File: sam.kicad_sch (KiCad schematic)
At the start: 23 parts, among them IC4 74ACT02, IC5 74ACT138, IC6 74ACT138N, J1 JTAG, J3 Conn_01x24, J4 Conn_01x24, U3 XC95144XL-TQ100, X1 14.31818MHz

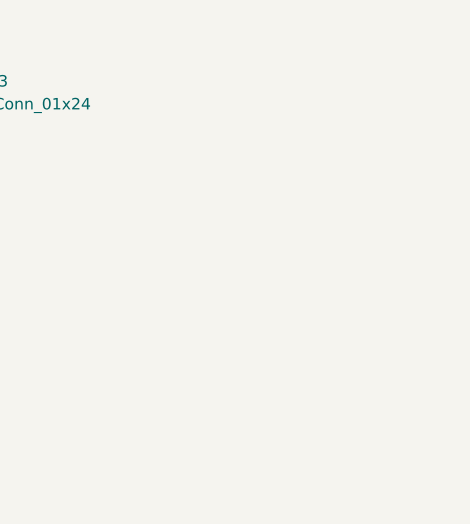
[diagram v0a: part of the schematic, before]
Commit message: progress routing
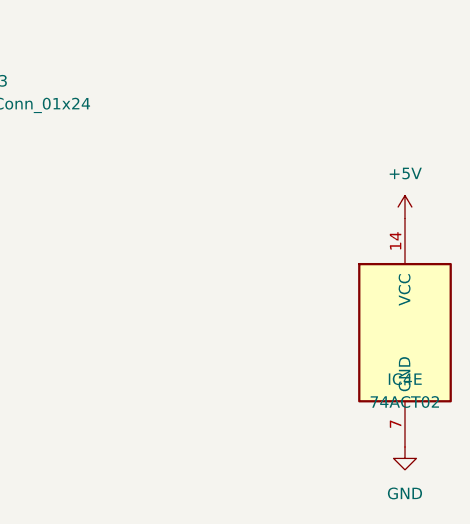
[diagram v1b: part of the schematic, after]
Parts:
- added unit 5 of IC4
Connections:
- net +5V: now also IC4.14 (VCC)
- net GND: now also IC4.7 (GND)
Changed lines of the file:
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@@
+	)
+	(symbol
+		(lib_id "74xx:74LS02")
+		(at 377.19 214.63 0)
+		(unit 5)
+		(exclude_from_sim no)
+		(in_bom yes)
+		(on_board yes)
+		(dnp no)
+		(property "Reference" "IC4"
+			(at 377.19 219.837 0)
+			(effects
+				(font
+					(size 1.27 1.27)
+				)
+			)
+		)
+		(property "Value" "74ACT02"
+			(at 377.19 222.377 0)
+			(effects
+				(font
+					(size 1.27 1.27)
+				)
+			)
+		)
+		(property "Footprint" "Package_SO:SOIC-14_3.9x8.7mm_P1.27mm"
+			(at 377.19 214.63 0)
+			(effects
+				(font
+					(size 1.27 1.27)
+				)
+				(hide yes)
+			)
+		)
+		(property "Datasheet" "http://www.ti.com/lit/gpn/sn74ls02"
+			(at 377.19 214.63 0)
+			(effects
+				(font
+					(size 1.27 1.27)
+				)
+				(hide yes)
+			)
+		)
+		(property "Description" ""
+			(at 377.19 214.63 0)
+			(effects
+				(font
+					(size 1.27 1.27)
+				)
+				(hide yes)
+			)
+		)
+		(property "DigiKey" "MC74ACT02DR2GOSCT-ND"
+			(at 377.19 214.63 0)
+			(effects
+				(font
+					(size 1.27 1.27)
+				)
+				(hide yes)
+			)
+		)
+		(property "SA2120" "Sheet 1 (spare)"
+			(at 377.19 214.63 0)
+			(effects
+				(font
+					(size 1.27 1.27)
+				)
+				(hide yes)
+			)
+		)
+		(pin "1"
+		)
+		(pin "2"
+		)
+		(pin "3"
+		)
+		(pin "4"
+		)
+		(pin "5"
+		)
+		(pin "6"
+		)
+		(pin "10"
+		)
+		(pin "8"
+		)
+		(pin "9"
+		)
+		(pin "11"
+		)
+		(pin "12"
+		)
+		(pin "13"
+		)
+		(pin "14"
+		)
+		(pin "7"
+		)
+		(instances
+			(project "DragonRevX4Plus"
+				(path "/280624a6-9139-42c2-8c41-e9b53b8715d2/c4b589a9-2d20-48b3-b81d-9e9e3aed36b4"
+					(reference "IC4")
+					(unit 5)
+				)
+			)
+		)
 	)
 	(symbol
@@
 	)
 	(symbol
+		(lib_id "power:+5V")
+		(at 377.19 201.93 0)
+		(unit 1)
+		(exclude_from_sim no)
+		(in_bom yes)
+		(on_board yes)
+		(dnp no)
+		(fields_autoplaced yes)
+		(property "Reference" "#PWR024"
+			(at 377.19 205.74 0)
+			(effects
+				(font
+					(size 1.27 1.27)
+				)
+				(hide yes)
+			)
+		)
+		(property "Value" "+5V"
+			(at 377.19 196.977 0)
+			(effects
+				(font
+					(size 1.27 1.27)
+				)
+			)
+		)
+		(property "Footprint" ""
+			(at 377.19 201.93 0)
+			(effects
+				(font
+					(size 1.27 1.27)
+				)
+				(hide yes)
+			)
+		)
+		(property "Datasheet" ""
+			(at 377.19 201.93 0)
+			(effects
+				(font
+					(size 1.27 1.27)
+				)
+				(hide yes)
+			)
+		)
+		(property "Description" ""
+			(at 377.19 201.93 0)
+			(effects
+				(font
+					(size 1.27 1.27)
+				)
+				(hide yes)
+			)
+		)
+		(pin "1"
+		)
+		(instances
+			(project "DragonRevX4Plus"
+				(path "/280624a6-9139-42c2-8c41-e9b53b8715d2/c4b589a9-2d20-48b3-b81d-9e9e3aed36b4"
+					(reference "#PWR024")
+					(unit 1)
+				)
+			)
+		)
+	)
+	(symbol
 		(lib_id "power:GND")
 		(at 228.6 50.8 0)
@@
 					(unit 1)
 				)
+			)
+		)
+	)
+	(symbol
+		(lib_id "power:GND")
+		(at 377.19 227.33 0)
+		(unit 1)
+		(exclude_from_sim no)
+		(in_bom yes)
+		(on_board yes)
+		(dnp no)
+		(fields_autoplaced yes)
+		(property "Reference" "#PWR025"
+			(at 377.19 233.68 0)
+			(effects
+				(font
+					(size 1.27 1.27)
+				)
+				(hide yes)
+			)
+		)
+		(property "Value" "GND"
+			(at 377.19 232.537 0)
+			(effects
+				(font
+					(size 1.27 1.27)
+				)
+			)
+		)
+		(property "Footprint" ""
+			(at 377.19 227.33 0)
+			(effects
+				(font
+					(size 1.27 1.27)
+				)
+				(hide yes)
+			)
+		)
+		(property "Datasheet" ""
+			(at 377.19 227.33 0)
+			(effects
+				(font
+					(size 1.27 1.27)
+				)
+				(hide yes)
+			)
+		)
+		(property "Description" ""
+			(at 377.19 227.33 0)
+			(effects
+				(font
+					(size 1.27 1.27)
+				)
+				(hide yes)
+			)
+		)
+		(pin "1"
+		)
+		(instances
+			(project "DragonRevX4Plus"
+				(path "/280624a6-9139-42c2-8c41-e9b53b8715d2/c4b589a9-2d20-48b3-b81d-9e9e3aed36b4"
+					(reference "#PWR025")
+					(unit 1)
+				)
